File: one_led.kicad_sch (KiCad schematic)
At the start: 2 parts

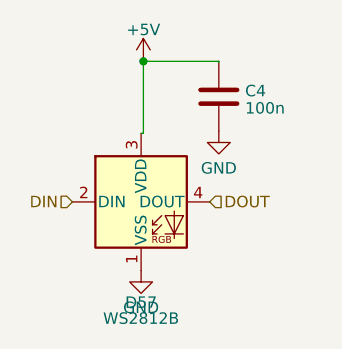
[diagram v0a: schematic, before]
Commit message: Publish the second iteration of the board
Squashed commit of the following:

commit 03137639306087c590cdda2dc88282cd072a3998
Author: IoT Maestro <iotmaestro@proton.me>
Date:   Wed Sep 20 22:36:39 2023 +0100

    Add JLCPCB PCBA files

commit 878c7d9bf7085809a9e5104ffe31423ea42c8531
Author: IoT Maestro <iotmaestro@proton.me>
Date:   Wed Sep 20 22:35:36 2023 +0100

    Got tired by committing everything one by one...

    Completed revision 2 including placements

commit 69d71586f674b78e869a3471f9a8dc84cc8d366e
Author: IoT Maestro <iotmaestro@proton.me>
Date:   Wed Sep 20 11:49:18 2023 +0100

    Made a few significant changes

     - removed individual channels per region, realistically it'll never be needed
     - added solder pads for all ESP32 pins

commit 97242618a214784a645288727facfb44c62f9649
Author: IoT Maestro <iotmaestro@proton.me>
Date:   Wed Sep 20 07:47:20 2023 +0100

    Assign footprints to components.

commit 45002d8314d0eb1705ebfe038861a6934b1b51b1
Author: IoT Maestro <iotmaestro@proton.me>
Date:   Wed Sep 20 07:42:14 2023 +0100

    Add an XT30 connector for power as well.

commit eac40f851972937518526a0ca66ce5db5aa91d03
Author: IoT Maestro <iotmaestro@proton.me>
Date:   Wed Sep 20 07:24:39 2023 +0100

    Sprinkle a few extra capacitors around for good measures

commit 3b0c2653f8ba452efb0d12ce280c7df2557f22ac
Author: IoT Maestro <iotmaestro@proton.me>
Date:   Wed Sep 20 07:24:15 2023 +0100

    Add .gitignore for backups

commit cc329acc9b2817cd8edc8902f09a11e0c2c65af4
Author: IoT Maestro <iotmaestro@proton.me>
Date:   Wed Sep 20 07:10:53 2023 +0100

    Updated the schematic

     - add 3V3-5V level shifters. This is not necessary but should improve signal integrity.
     - add a series resistor for data lines. Likewise it's not 100% necessary but improves signal integrity and eliminates ringing
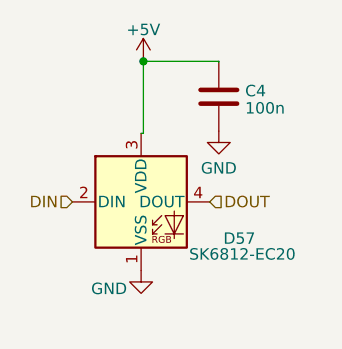
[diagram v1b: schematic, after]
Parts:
- C4: footprint Capacitor_SMD:C_0402_1005Metric -> Capacitor_SMD:C_0603_1608Metric; JLCPCB_PART C1525 -> C14663
- D57: value WS2812B -> SK6812-EC20; footprint mapacr:XL-2121RGBC-WS2812B -> mapacr:LED_SK6812-EC20; symbol mapacr:XL-2121RGBC-WS2812B -> mapacr:SK6812-EC20; JLCPCB_PART C5349957 -> C2909058
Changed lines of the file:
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@@
     (effects (font (size 1.27 1.27)) (justify left))
   )
-  (symbol (lib_id "mapacr:XL-2121RGBC-WS2812B") (at 89.154 66.548 0) (unit 1)
+  (symbol (lib_id "mapacr:SK6812-EC20") (at 89.154 66.548 0) (unit 1)
     (in_bom yes) (on_board yes) (dnp no)
-    (property "Reference" "D57" (at 89.154 77.724 0)
-      (effects (font (size 1.27 1.27)))
-    )
-    (property "Value" "WS2812B" (at 89.154 79.502 0)
-      (effects (font (size 1.27 1.27)))
-    )
-    (property "Footprint" "mapacr:XL-2121RGBC-WS2812B" (at 90.424 74.168 0)
+    (property "Reference" "D57" (at 100.076 70.612 0)
+      (effects (font (size 1.27 1.27)))
+    )
+    (property "Value" "SK6812-EC20" (at 94.488 71.628 0)
+      (effects (font (size 1.27 1.27)) (justify left top))
+    )
+    (property "Footprint" "mapacr:LED_SK6812-EC20" (at 90.424 74.168 0)
       (effects (font (size 1.27 1.27)) (justify left top) hide)
     )
-    (property "Datasheet" "https://datasheet.lcsc.com/lcsc/2301111010_XINGLIGHT-XL-2121RGBC-WS2812B_C5349957.pdf" (at 91.694 76.073 0)
+    (property "Datasheet" "https://datasheet.lcsc.com/lcsc/2110250930_OPSCO-Optoelectronics-SK6812-EC20_C2909058.pdf" (at 91.694 76.073 0)
       (effects (font (size 1.27 1.27)) (justify left top) hide)
     )
-    (property "JLCPCB_PART" "C5349957" (at 89.154 66.548 0)
+    (property "JLCPCB_PART" "C2909058" (at 98.044 79.248 0)
       (effects (font (size 1.27 1.27)) hide)
     )
@@
       (effects (font (size 1.27 1.27)) (justify left))
     )
-    (property "Footprint" "Capacitor_SMD:C_0402_1005Metric" (at 98.7552 58.674 0)
+    (property "Footprint" "Capacitor_SMD:C_0603_1608Metric" (at 98.7552 58.674 0)
       (effects (font (size 1.27 1.27)) hide)
     )
@@
       (effects (font (size 1.27 1.27)) hide)
     )
-    (property "JLCPCB_PART" "C1525" (at 97.79 54.864 0)
+    (property "JLCPCB_PART" "C14663" (at 97.79 54.864 0)
       (effects (font (size 1.27 1.27)) hide)
     )
@@
   )
   (symbol (lib_id "power:GND") (at 89.154 74.168 0) (unit 1)
-    (in_bom yes) (on_board yes) (dnp no) (fields_autoplaced)
+    (in_bom yes) (on_board yes) (dnp no)
     (property "Reference" "#PWR016" (at 89.154 80.518 0)
       (effects (font (size 1.27 1.27)) hide)
     )
-    (property "Value" "GND" (at 89.154 78.3035 0)
-      (effects (font (size 1.27 1.27)))
-    )
+    (property "Value" "GND" (at 85.598 76.2 0)
+      (effects (font (size 1.27 1.27)))
+    )
